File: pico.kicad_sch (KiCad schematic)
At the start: 54 parts, among them J1 Jack 3.5mm, J12 SWD, J14 JST PH 4, J15 LCD left, J17 LCD right, J2 DIN5, J25 JST PH 3, J26 JST PH 3, J3 Jack 3.5mm, J4 DIN5, J5 Jack 6.35mm, J8 Jack 6.35mm, SW1 24P/R 24mm, SW10 Momentary switch, SW2 24P/R 24mm, SW3 Micro Button, SW4 Micro Button, SW5 Momentary switch, SW6 Momentary switch, SW7 Momentary switch, SW8 Momentary switch, SW9 Momentary switch, U12 AT24CS01-STUM, U2 TLP2761, U3 STM32G0B1CET6

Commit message: small edits
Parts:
- D1: footprint Diode_SMD:D_SOD-123F -> Diode_SMD:D_SOD-123
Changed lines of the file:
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@@
 			)
 		)
-		(property "Footprint" "Diode_SMD:D_SOD-123F"
+		(property "Footprint" "Diode_SMD:D_SOD-123"
 			(at 54.61 80.01 0)
 			(hide yes)

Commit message: a few edits
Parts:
- SW3: Notes Boot -> Firmware DFU request - requires working firmware, use SWD f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
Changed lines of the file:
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@@
 			)
 		)
-		(property "Notes" "Boot"
+		(property "Notes" "Firmware DFU request - requires working firmware, use SWD for recovery"
 			(at 99.06 96.52 0)
 			(hide yes)

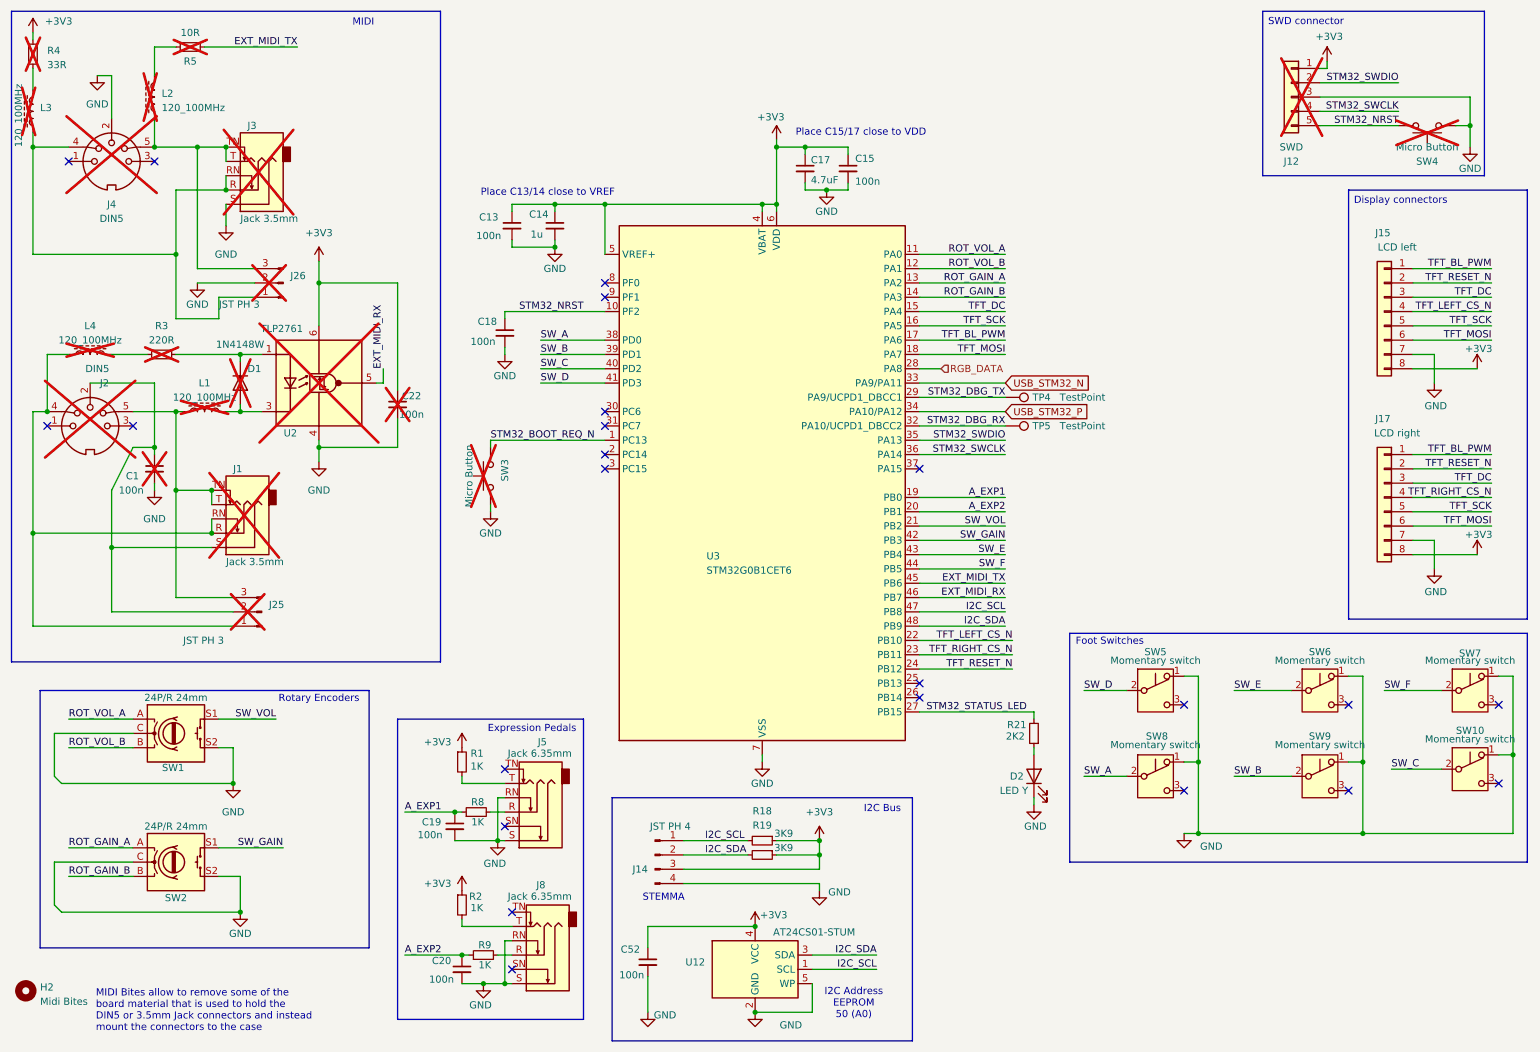
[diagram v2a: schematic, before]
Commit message: fixed warnings.
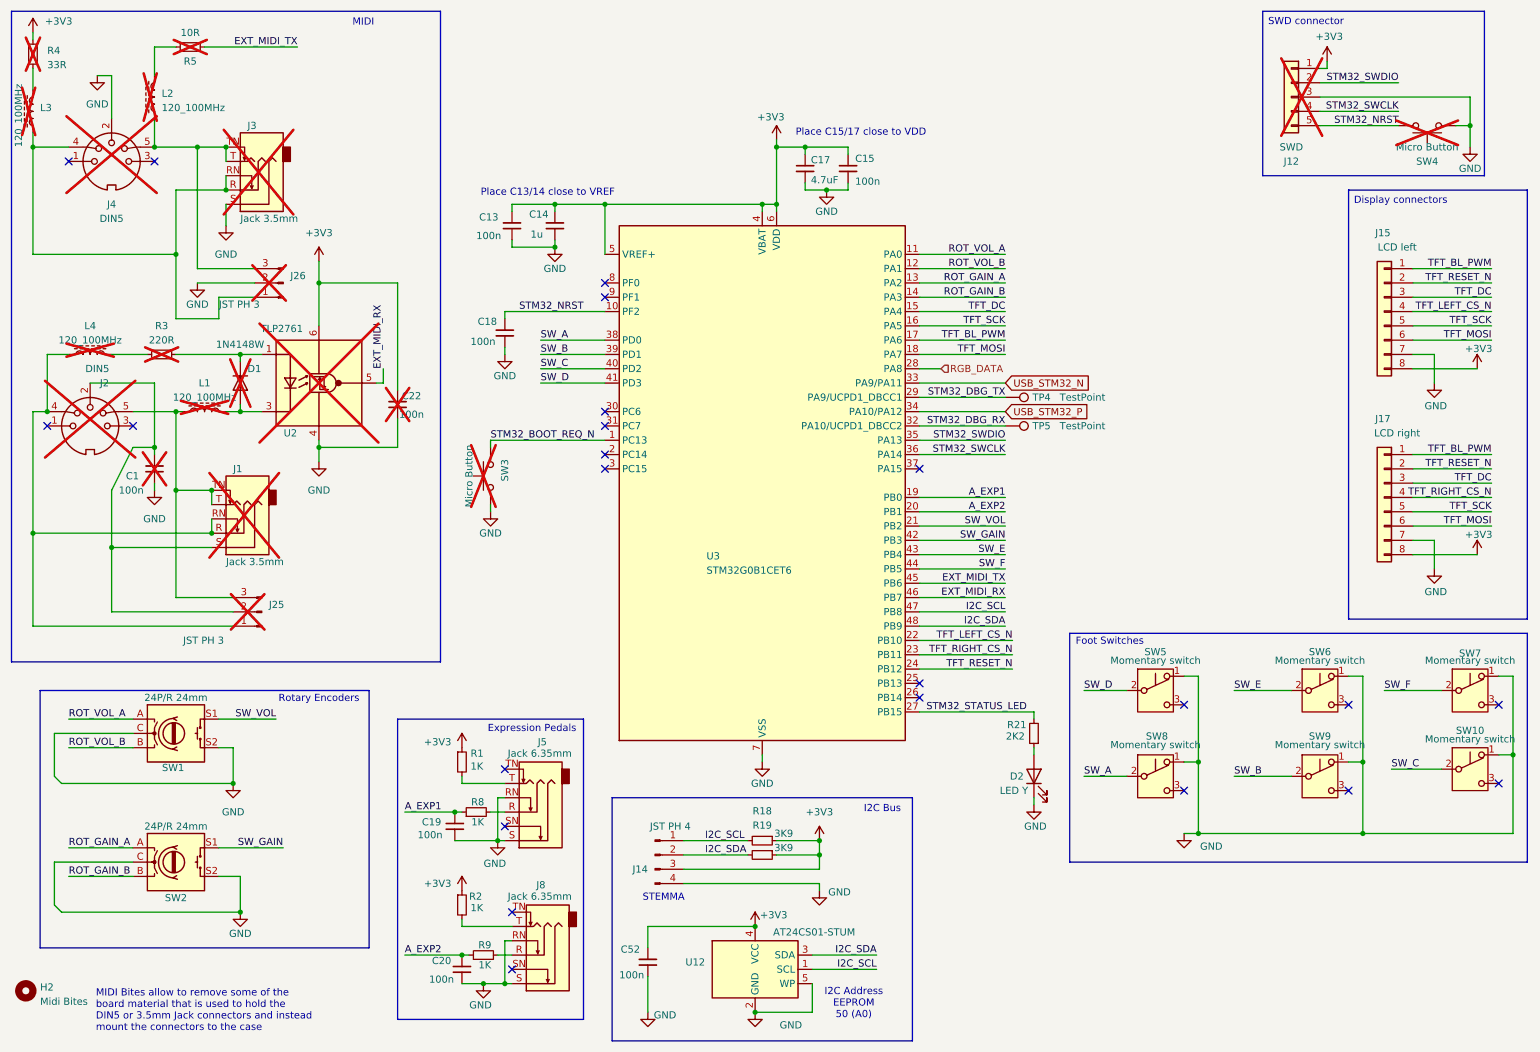
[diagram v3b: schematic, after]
